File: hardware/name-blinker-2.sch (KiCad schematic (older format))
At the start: 40 parts, among them M1 MOUNTING-HOLE, M10 MOUNTING-HOLE, M12 MOUNTING-HOLE, M13 MOUNTING-HOLE, M2 MOUNTING-HOLE, M3 MOUNTING-HOLE, M4 MOUNTING-HOLE, M5 MOUNTING-HOLE, M6 MOUNTING-HOLE, M7 MOUNTING-HOLE, M8 MOUNTING-HOLE, M9 MOUNTING-HOLE, P1 CONN_01X08, P2 USB_OTG, SW2 SMD-TOGGLE-SWITCH-2CH_2X3P-7X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, U1 MCP73831, U2 BMD-300, U3 TPS63051

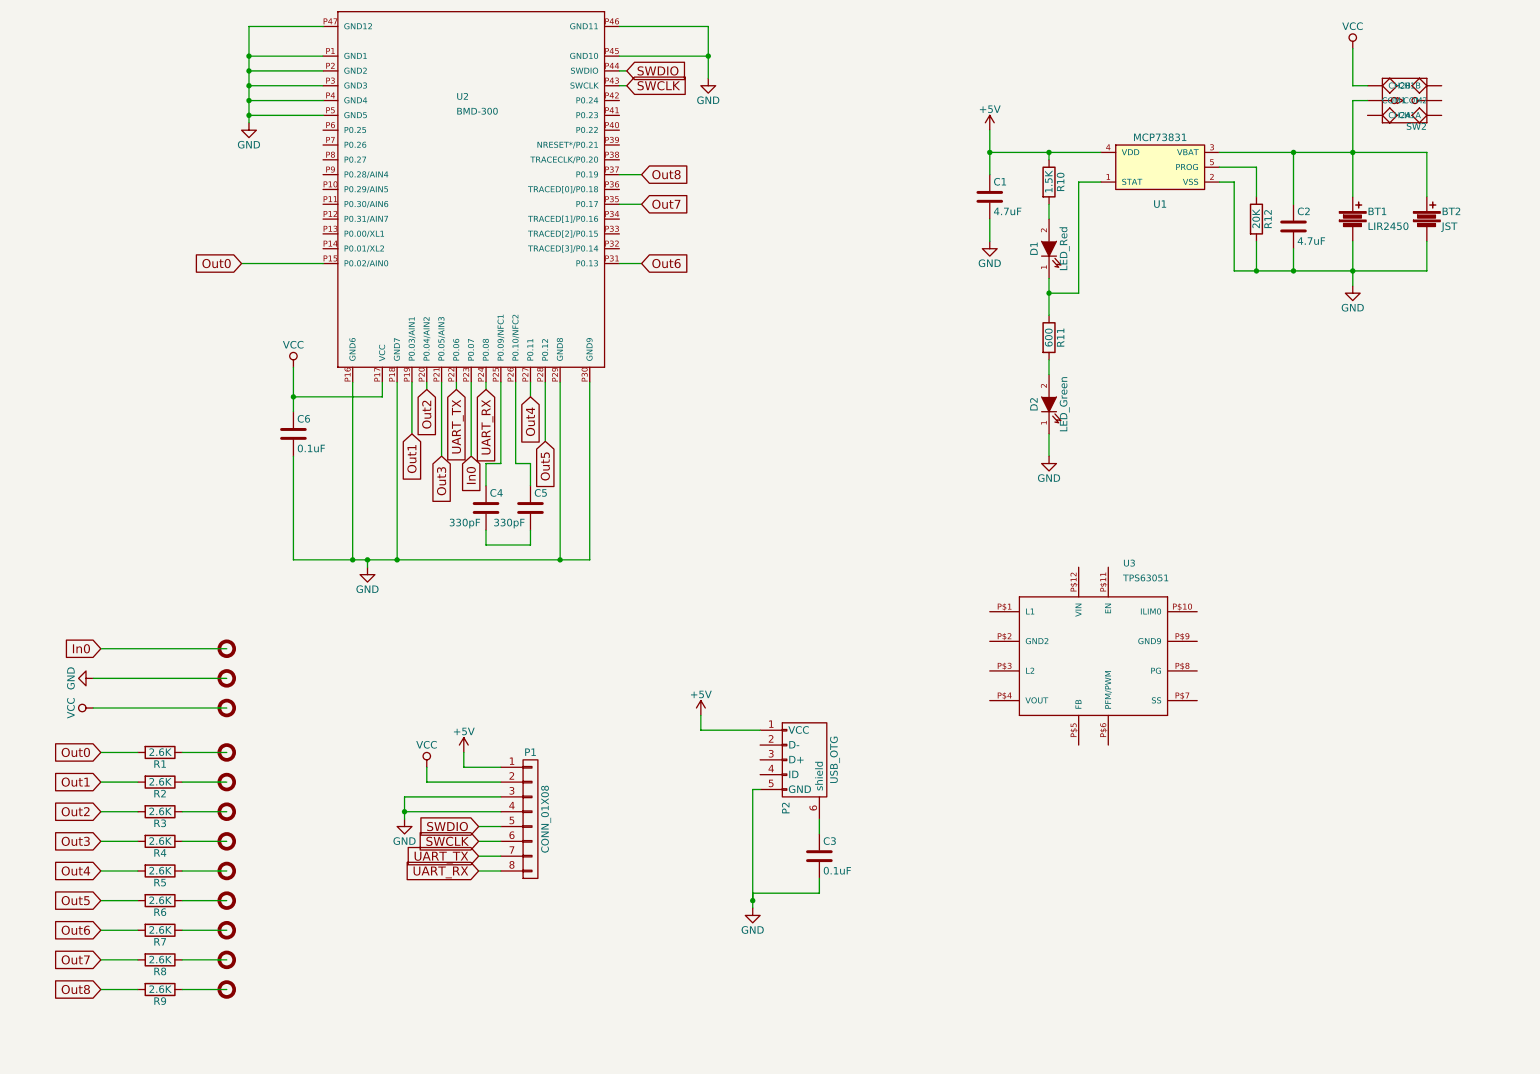
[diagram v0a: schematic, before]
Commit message: adjusted sch
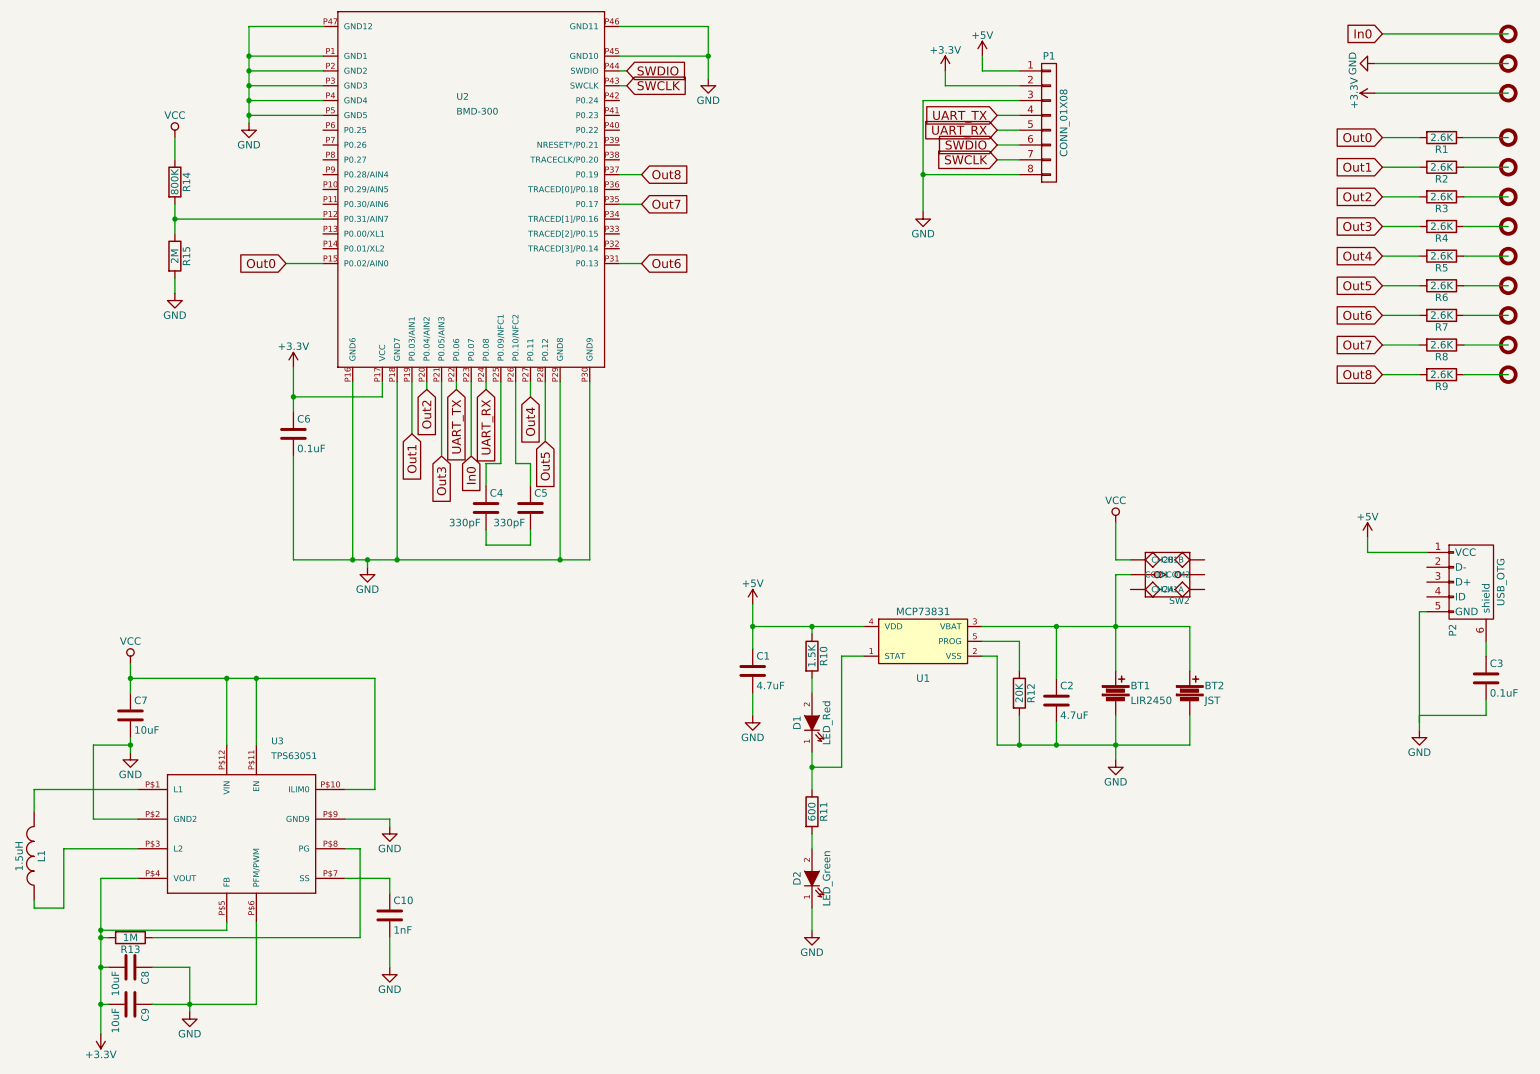
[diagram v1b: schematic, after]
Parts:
- added C10: 1nF, symbol C
- added C7: 10uF, Capacitors_SMD:c_elec_4x5.8, symbol C
- added C8, C9: 10uF, symbol C
- added L1: 1.5uH, symbol INDUCTOR
- added R13: 1M, symbol R
- added R14: 800K, symbol R
- added R15: 2M, symbol R
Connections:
- net GND: now also P1.8 (P8), U3.P$2 (GND2), U3.P$6 (PFM/PWM), U3.P$9 (GND9), C10.2, C7.2, C8.1, C9.1, R15.2; no longer P1.4 (P4)
- net SWCLK: now also P1.7 (P7); no longer P1.6 (P6)
- net SWDIO: now also P1.6 (P6); no longer P1.5 (P5)
- net UART_RX: now also P1.5 (P5); no longer P1.8 (P8)
- net UART_TX: now also P1.4 (P4); no longer P1.7 (P7)
- net VCC: now also U3.P$10 (ILIM0), U3.P$11 (EN), U3.P$12 (VIN), C7.1, R14.1; no longer C6.1, M12.1, P1.2 (P2), U2.P17 (VCC)
- net at U2.P12 (P0.31/AIN7): now also R14.2, R15.1
- net at U3.P$1 (L1): now also L1.2
- net at U3.P$3 (L2): now also L1.1
- net +3V3: now reaches U3.P$4 (VOUT)
- net +3V3: now also C6.1, M12.1, P1.2 (P2), U2.P17 (VCC), U3.P$5 (FB), C8.2, C9.2, R13.2
- net at U3.P$7 (SS): now also C10.1
- net at U3.P$8 (PG): now also R13.1
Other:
- moved on the sheet: BT1, BT2, C1, C2, C3, D1, D2, P1, P2, R1, R10, R11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
